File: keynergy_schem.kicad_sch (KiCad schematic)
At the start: 40 parts, among them J1 Conn_01x04_Pin, J2 Conn_01x04_Pin, J3 Conn_01x02_Pin, J4 Conn_01x04_Pin, J5 Conn_01x04_Pin, J6 Conn_01x04_Pin

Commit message: new updates
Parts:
- added J7: Conn_01x04_Pin, Connector_PinHeader_2.54mm:PinHeader_1x04_P2.54mm_Vertical, symbol Connector:Conn_01x04_Pin
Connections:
- net Column 1: now also J7.1 (Pin_1)
- net Column 2: now also J7.2 (Pin_2)
- net Column 3: now also J7.3 (Pin_3)
- net Column 4: now also J7.4 (Pin_4)
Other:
- note added: "PCB 2"
- moved on the sheet: C2, D1, D2, D3, D4, K10, K11, K12, K13, K14, K15, K16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

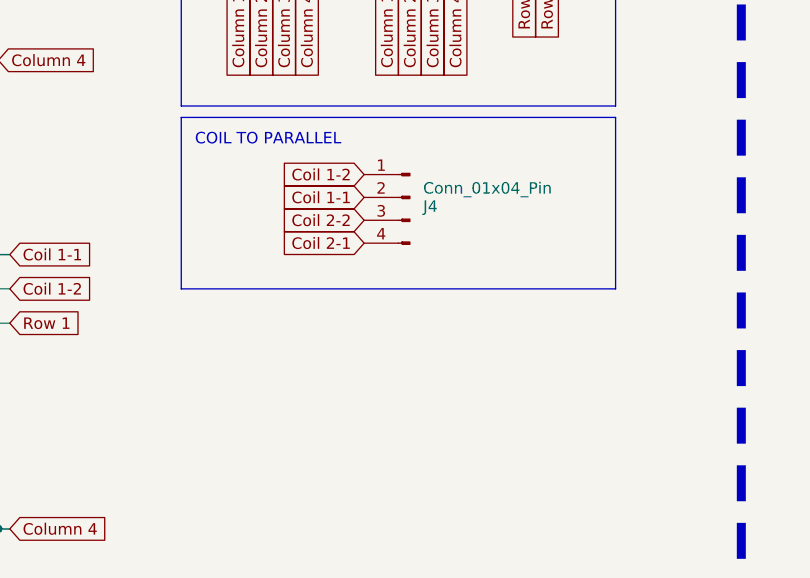
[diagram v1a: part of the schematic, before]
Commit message: new updates, pdf exported
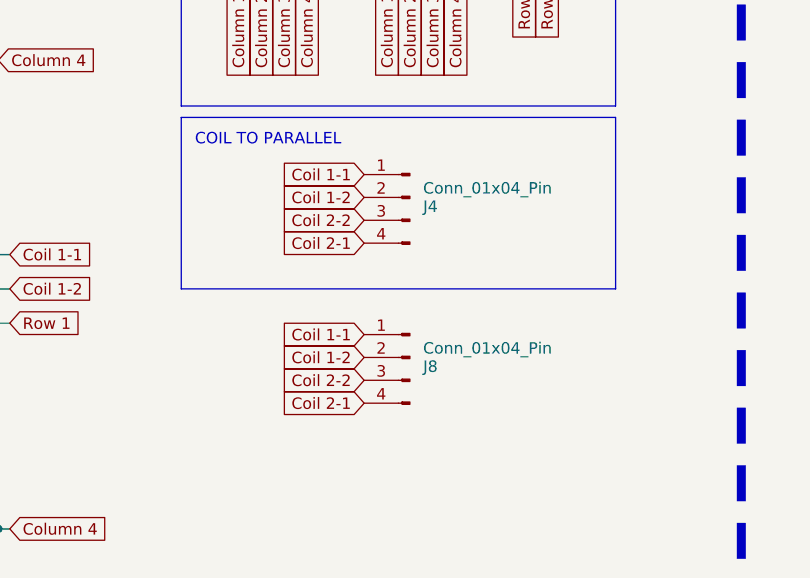
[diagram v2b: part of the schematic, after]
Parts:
- added J8: Conn_01x04_Pin, Connector_PinHeader_2.54mm:PinHeader_1x04_P2.54mm_Vertical, symbol Connector:Conn_01x04_Pin
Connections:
- net Coil 1-1: now also J4.1 (Pin_1), J8.1 (Pin_1); no longer J4.2 (Pin_2)
- net Coil 1-2: now also J4.2 (Pin_2), J8.2 (Pin_2); no longer J4.1 (Pin_1)
- net Coil 2-1: now also J8.4 (Pin_4)
- net Coil 2-2: now also J8.3 (Pin_3)

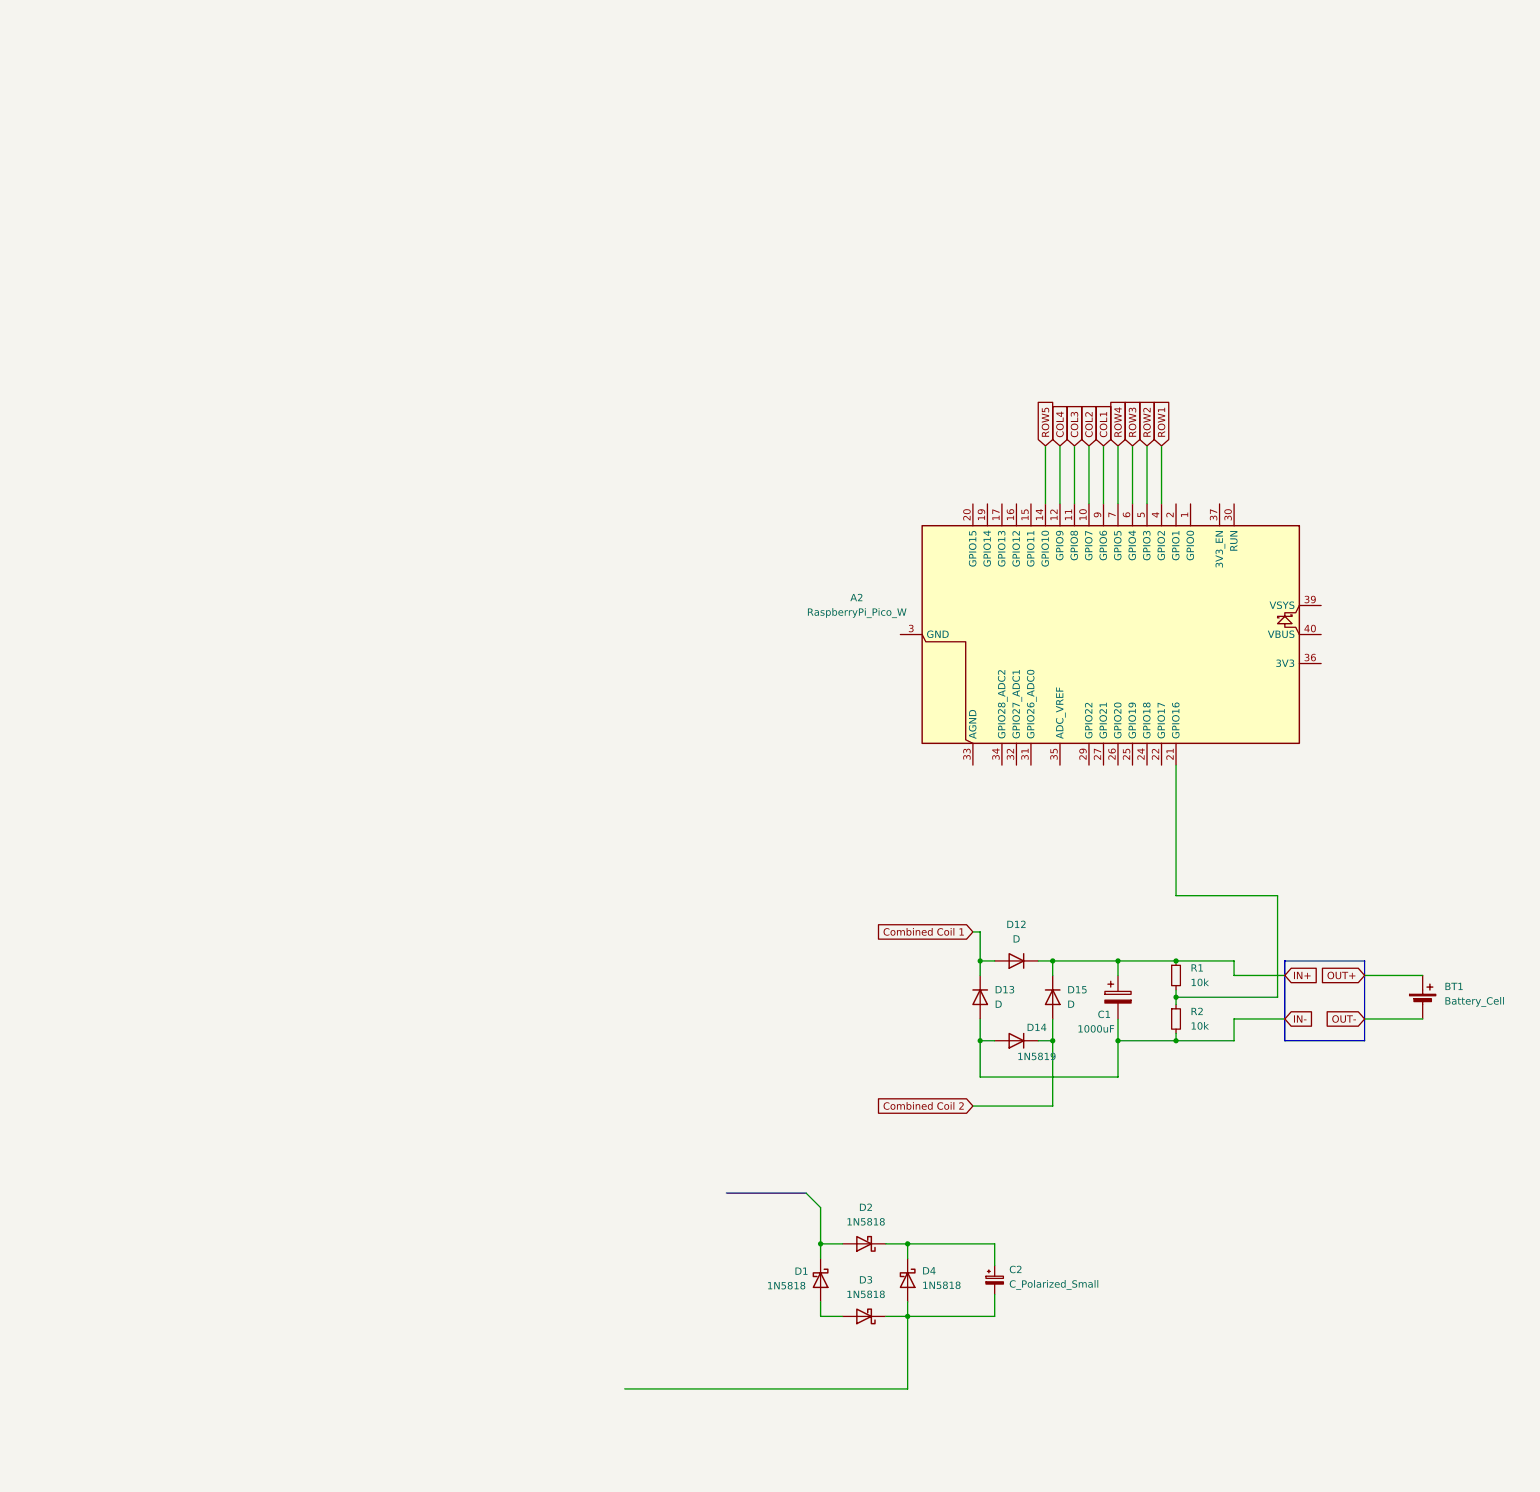
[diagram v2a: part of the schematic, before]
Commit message: new updates
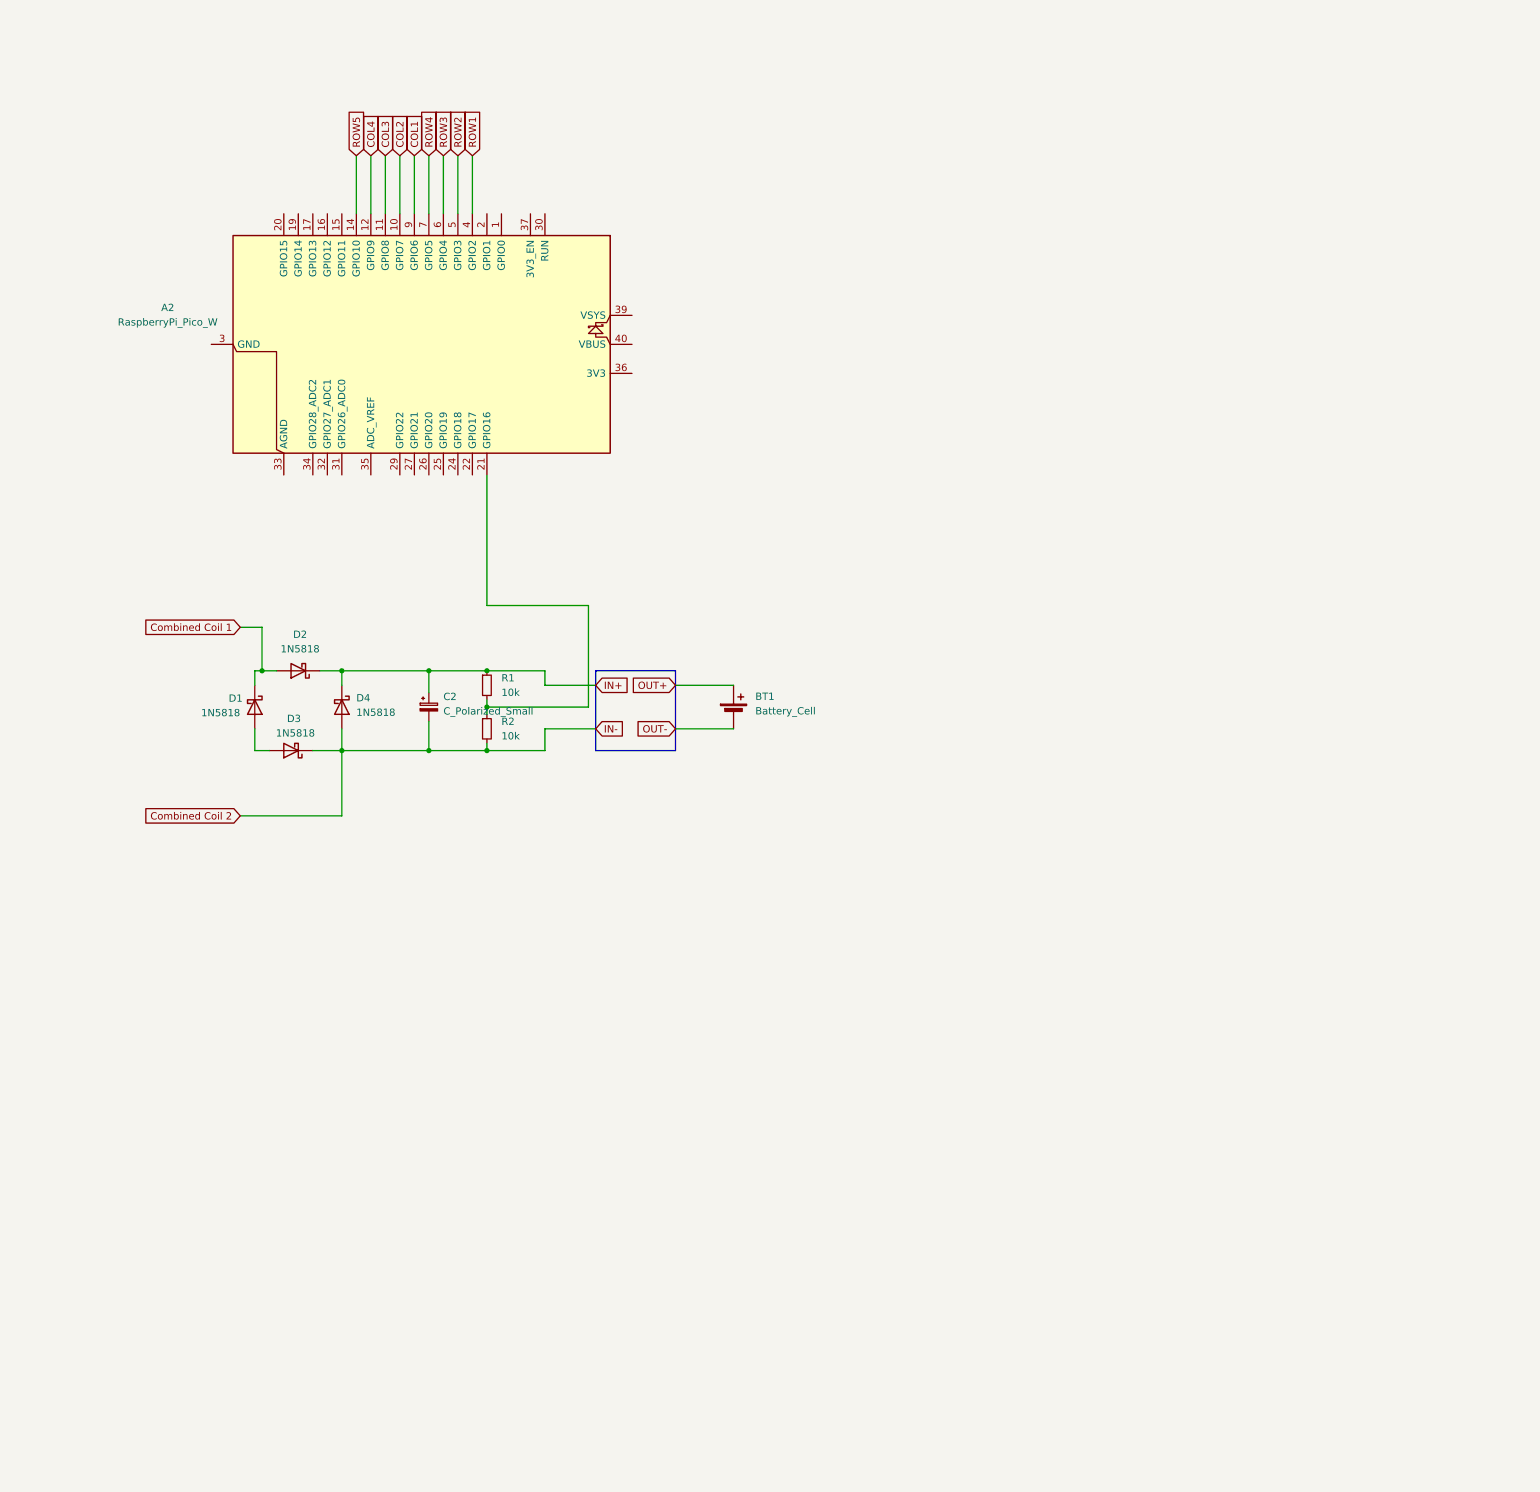
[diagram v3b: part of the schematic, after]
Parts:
- removed C1: 1000uF, Capacitor_THT:CP_Radial_D8.0mm_P5.00mm, symbol Device:C_Polarized
- removed D12, D13, D15: D, Diode_THT:D_DO-34_SOD68_P7.62mm_Horizontal, symbol Device:D
- removed D14: 1N5819, Diode_THT:D_DO-34_SOD68_P7.62mm_Horizontal, symbol Device:D
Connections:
- net IN- is gone; now on net Combined Coil 2: R2.2
- net Combined Coil 1: now also D1.1 (K), D2.2 (A)
- net Combined Coil 2: now also C2.2, D3.1 (K), D4.2 (A)
- net IN+: now also C2.1, D2.1 (K), D4.1 (K)
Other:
- moved on the sheet: A2, BT1, C2, D1, D2, D3, D4, R1, R2

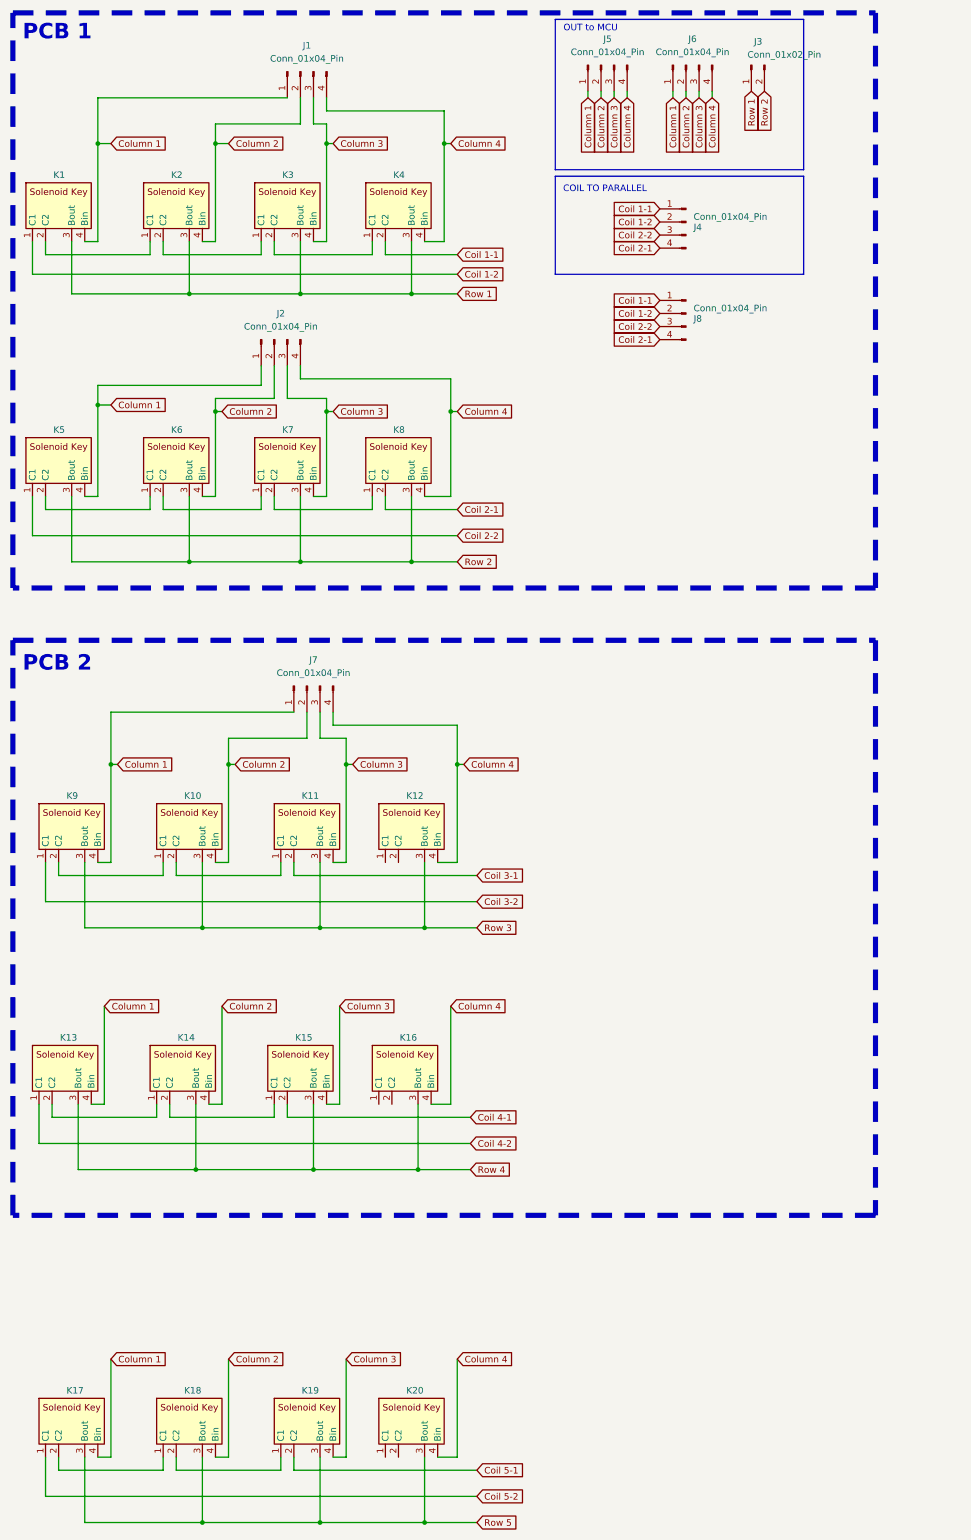
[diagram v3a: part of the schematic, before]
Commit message: updated
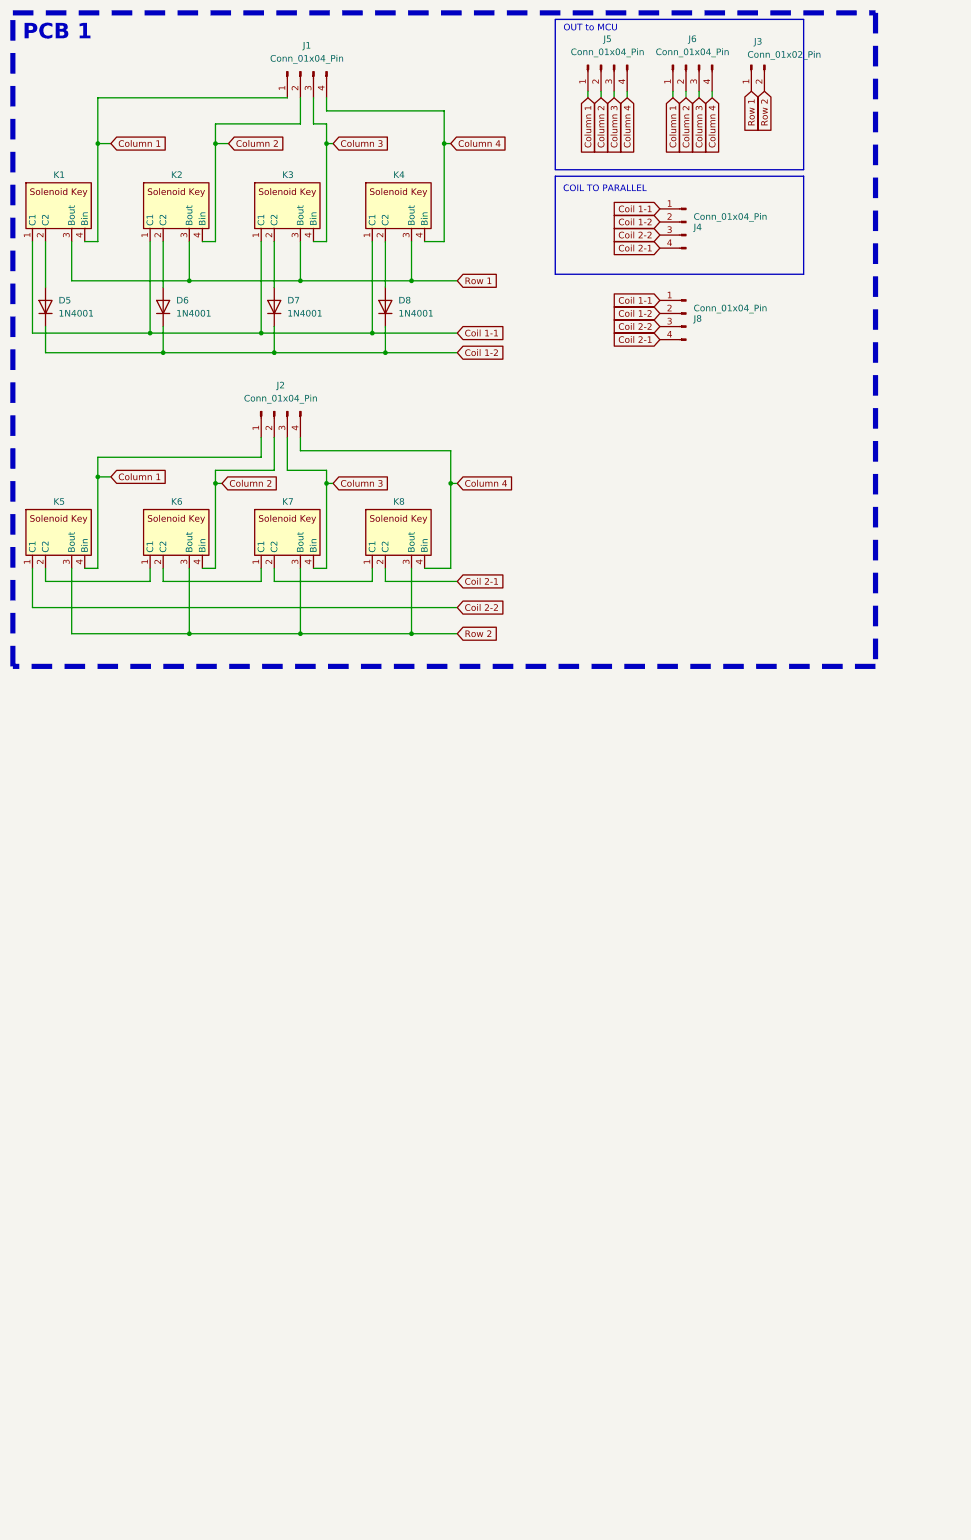
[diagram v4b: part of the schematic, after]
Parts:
- removed J7: Conn_01x04_Pin, Connector_PinHeader_2.54mm:PinHeader_1x04_P2.54mm_Vertical, symbol Connector:Conn_01x04_Pin
- removed K10, K11, K12, K13, K14, K15, K16, K17, K18, K19, K20, K9: ~, project library:Solenoid Key, symbol Key_symbol:Solenoid_Key
- added D5, D6, D7, D8: 1N4001, Diode_THT:D_DO-34_SOD68_P7.62mm_Horizontal, symbol Device:D
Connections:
- net Coil 1-1: now also K1.1 (C1), K2.1 (C1), K3.1 (C1), K4.1 (C1); no longer K4.2 (C2)
- net Coil 1-2: now also D5.1 (K), D6.1 (K), D7.1 (K), D8.1 (K); no longer K1.1 (C1)
- net at K2.2 (C2): now also D6.2 (A); no longer K3.1 (C1)
- net at K3.2 (C2): now also D7.2 (A); no longer K4.1 (C1)
- net at K1.2 (C2): now also D5.2 (A); no longer K2.1 (C1)
- new net: D8.2 (A), K4.2 (C2)
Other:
- note removed: "PCB 2"
- moved on the sheet: J2, K5, K6, K7, K8
